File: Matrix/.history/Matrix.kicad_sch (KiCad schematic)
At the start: 1 part

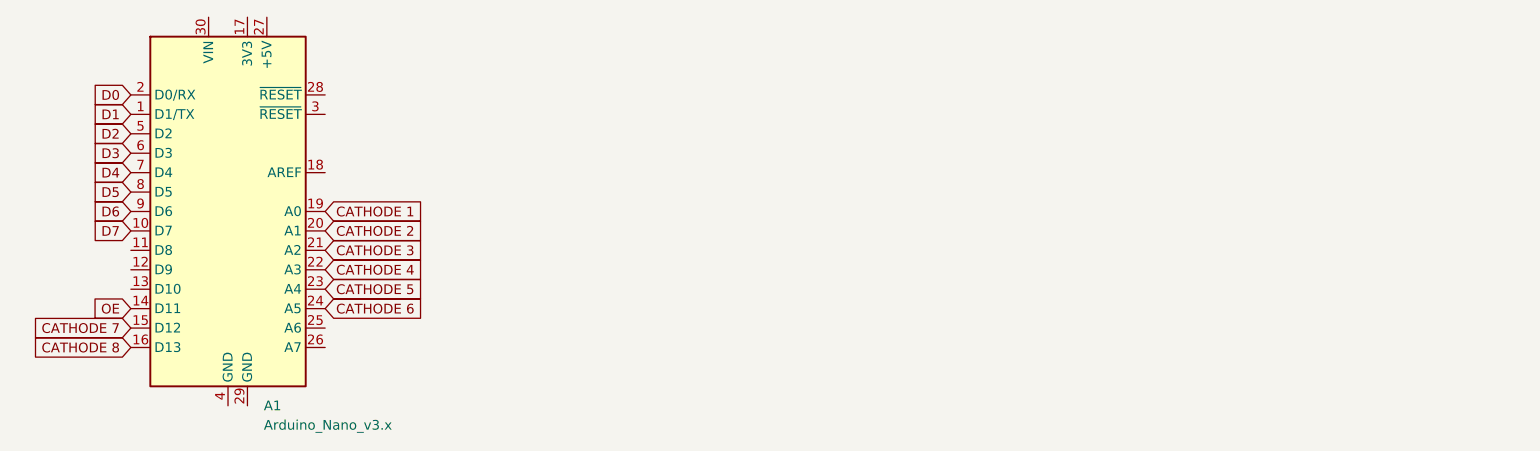
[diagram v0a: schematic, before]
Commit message: Update Matrix.kicad_sch
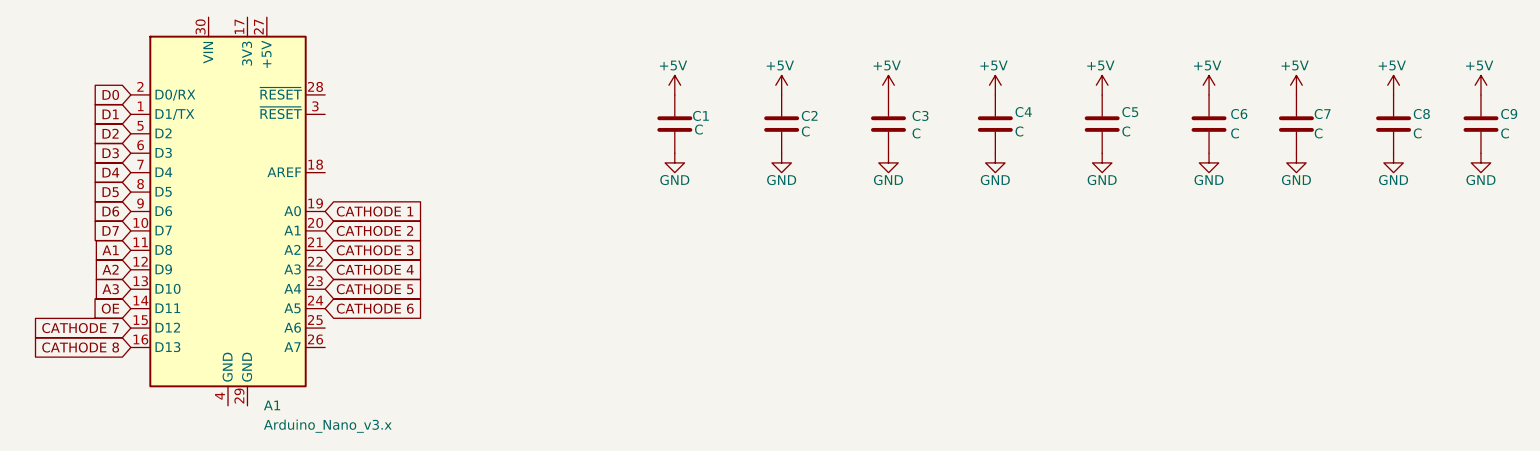
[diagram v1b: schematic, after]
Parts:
- added C1, C2, C3, C4, C5, C6, C7, C8, C9: C, symbol Device:C
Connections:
- net A1: now reaches A1.11 (D8)
- net A2: now reaches A1.12 (D9)
- net A3: now reaches A1.13 (D10)
- new net +5V: C1.1, C2.1, C3.1, C4.1, C5.1, C6.1, C7.1, C8.1, C9.1
- new net GND: C1.2, C2.2, C3.2, C4.2, C5.2, C6.2, C7.2, C8.2, C9.2
